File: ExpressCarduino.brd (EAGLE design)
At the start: 38.8 x 27.7 mm, 14 parts, among them IC1 MCP23017ML, U1 AP3012

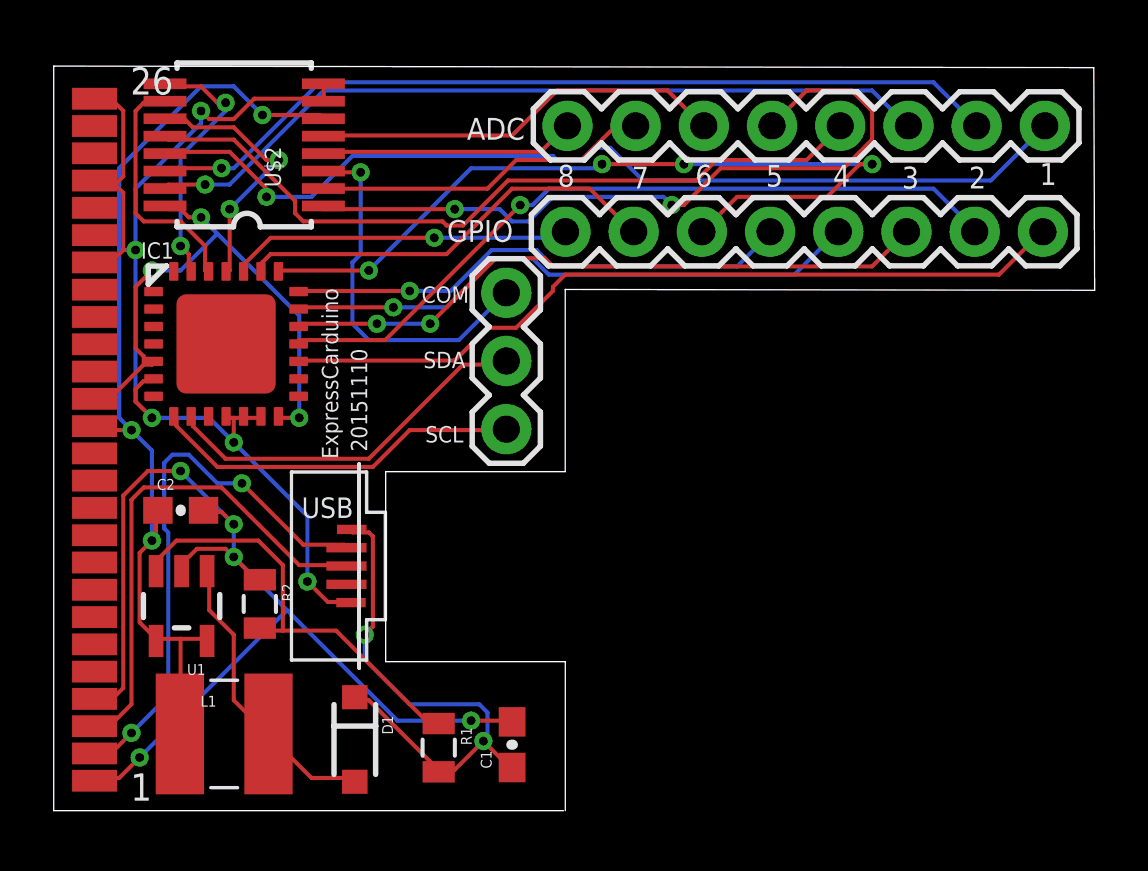
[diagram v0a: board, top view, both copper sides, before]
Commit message: I keep tweaking the board...
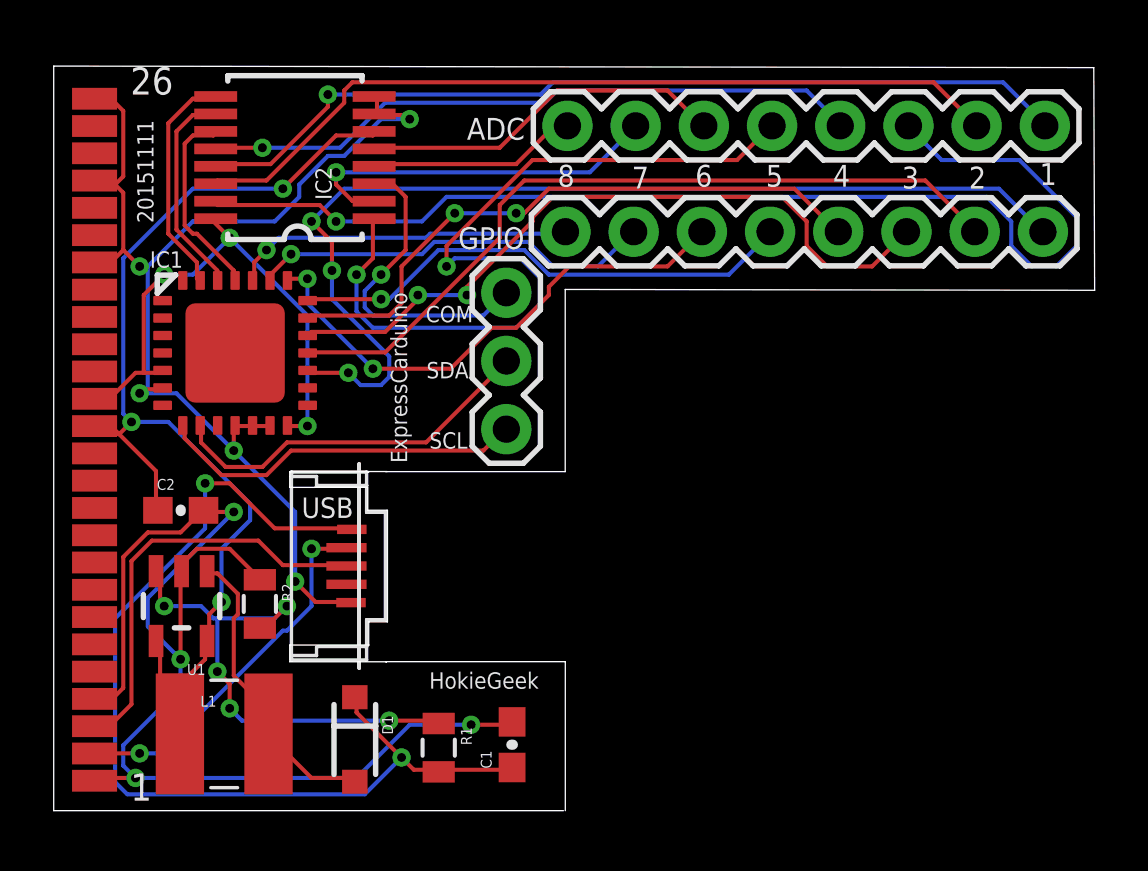
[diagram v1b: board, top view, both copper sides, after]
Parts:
- removed U$2: SN74LV4051A, HokieGeek:TSSOP16
- added IC2: SN74LV4051A, HokieGeek:TSSOP16
- moved IC1 0.48 mm to (6.76, 17.0)
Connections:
- net GND: now also IC2.7, IC2.8; no longer U$2.7, U$2.8
- net MUX_A: now also IC2.11; no longer U$2.11
- net MUX_B: now also IC2.10; no longer U$2.10
- net MUX_C: now also IC2.9; no longer U$2.9
- net MUX_COM: now also IC2.3; no longer U$2.3
- net N$19: now also IC2.13; no longer U$2.13
- net N$20: now also IC2.14; no longer U$2.14
- net N$21: now also IC2.15; no longer U$2.15
- net N$22: now also IC2.12; no longer U$2.12
- net N$23: now also IC2.1; no longer U$2.1
- net N$24: now also IC2.5; no longer U$2.5
- net N$25: now also IC2.2; no longer U$2.2
- net N$26: now also IC2.4; no longer U$2.4
- net VCC: now also IC2.16; no longer U$2.16
- net VUSB: now also IC2.6; no longer U$2.6
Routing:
- net 9V: track 20.2 -> 37.5 mm
- net N$21: track 29.7 -> 43.5 mm
- net N$8: track 31.2 -> 19.7 mm, vias 4 -> 2
- net N$2: track 29.8 -> 38.8 mm, vias 0 -> 3
- net USBD-: track 20.7 -> 13.8 mm
- net VUSB: track 36.2 -> 43.1 mm
- net GND_USB: track 43.1 -> 47.6 mm, vias 5 -> 4
- net N$22: track 28.3 -> 24.7 mm, vias 0 -> 1
- net N$1: track 16.4 -> 19.4 mm, vias 0 -> 5
- net USBD+: track 18.8 -> 15.8 mm
- net N$23: track 27.9 -> 30.8 mm
- net N$19: track 35.9 -> 33.2 mm
- net MUX_A: track 9.88 -> 7.33 mm, vias 2 -> 0
- net N$5: track 24.4 -> 26.9 mm
- net MUX_COM: track 13.9 -> 11.9 mm
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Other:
- outline, holes or cut-outs redrawn
- board text added: "20151111"
- board text added: "HokieGeek"
- board text removed: "20151110"
